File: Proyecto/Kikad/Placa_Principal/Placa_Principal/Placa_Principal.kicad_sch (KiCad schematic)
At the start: 9 parts, among them J1 Screw_Terminal_01x03, J2 Screw_Terminal_01x03, J3 Screw_Terminal_01x03, J4 Screw_Terminal_01x03, J5 USB_C_Receptacle_PowerOnly_6P, J6 Screw_Terminal_01x07, SW1 SW_DIP_x01, U1 ESP32-DEVKITC-32D

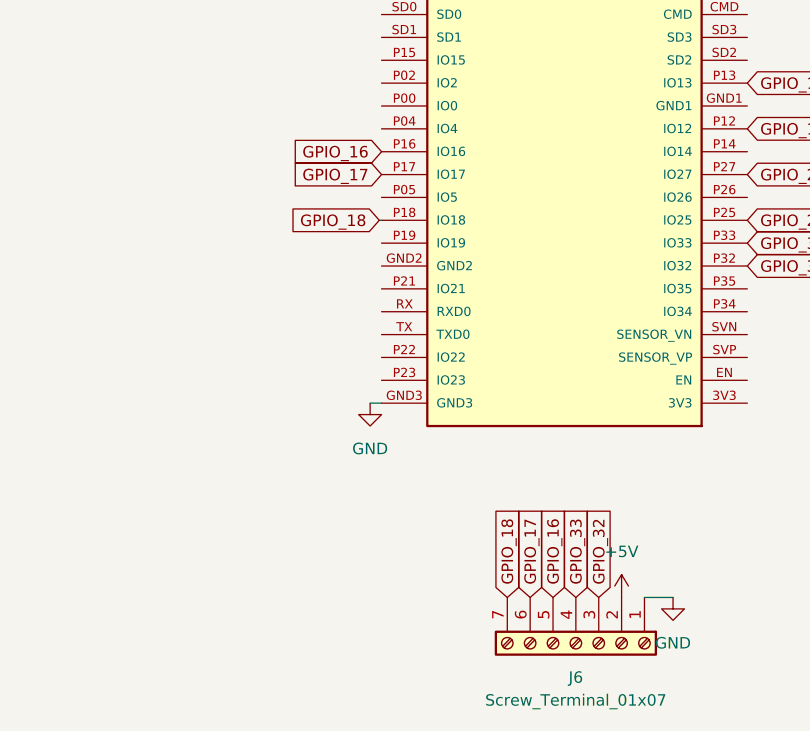
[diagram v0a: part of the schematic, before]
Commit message: Cambie 2 gpio
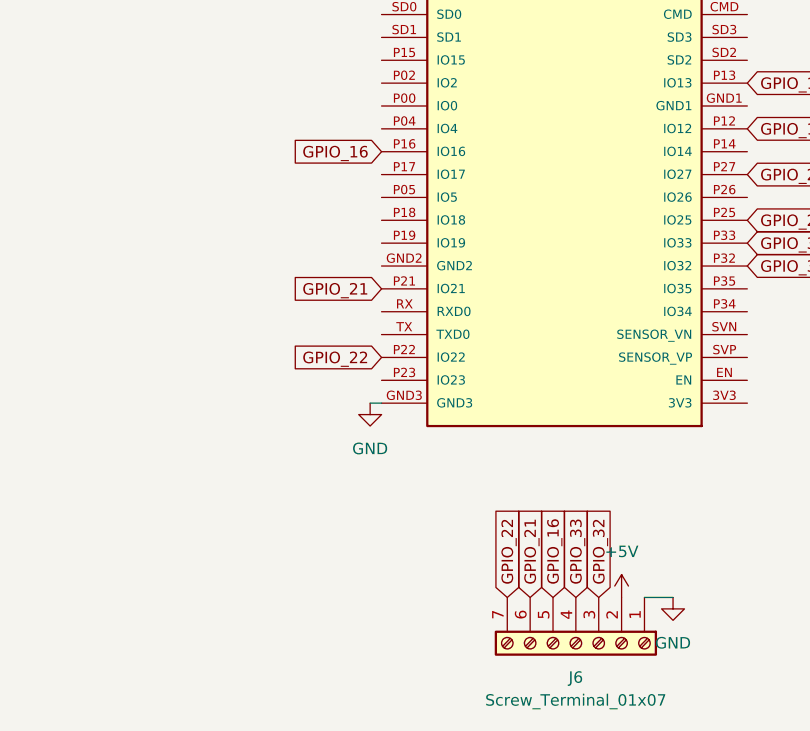
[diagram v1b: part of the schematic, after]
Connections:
- net GPIO_21: now reaches U1.P21 (IO21)
- net GPIO_21: now also J6.6 (Pin_6)
- net GPIO_22: now reaches U1.P22 (IO22)
- net GPIO_22: now also J6.7 (Pin_7)
- net GPIO_17: no longer names the net of U1.P17 (IO17)
- net GPIO_17: no longer J6.6 (Pin_6)
- net GPIO_18: no longer names the net of U1.P18 (IO18)
- net GPIO_18: no longer J6.7 (Pin_7)
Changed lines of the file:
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@@
 	(wire
 		(pts
-			(xy 150.876 106.68) (xy 151.13 106.68)
+			(xy 180.34 148.59) (xy 183.515 148.59)
 		)
 		(stroke
@@
 	(wire
 		(pts
-			(xy 180.34 148.59) (xy 183.515 148.59)
+			(xy 93.98 111.76) (xy 93.98 111.125)
 		)
 		(stroke
@@
 		)
 	)
-	(wire
-		(pts
-			(xy 93.98 111.76) (xy 93.98 111.125)
-		)
-		(stroke
-			(width 0)
-			(type default)
-		)
-	)
 	(global_label "GPIO_12"
 		(shape input)
@@
 		)
 	)
-	(global_label "GPIO_17"
+	(global_label "GPIO_21"
 		(shape input)
 		(at 167.64 148.59 90)
@@
 		)
 	)
-	(global_label "GPIO_18"
+	(global_label "GPIO_22"
 		(shape input)
 		(at 165.1 148.59 90)
@@
 		)
 	)
-	(global_label "GPIO_18"
-		(shape input)
-		(at 150.876 106.68 180)
-		(fields_autoplaced yes)
-		(effects
-			(font
-				(size 1.27 1.27)
-			)
-			(justify right)
-		)
-		(property "Intersheetrefs" "${INTERSHEET_REFS}"
-			(at 140.0289 106.68 0)
+	(global_label "GPIO_22"
+		(shape input)
+		(at 151.13 121.92 180)
+		(fields_autoplaced yes)
+		(effects
+			(font
+				(size 1.27 1.27)
+			)
+			(justify right)
+		)
+		(property "Intersheetrefs" "${INTERSHEET_REFS}"
+			(at 140.2829 121.92 0)
 			(effects
 				(font
@@
 		)
 	)
-	(global_label "GPIO_17"
-		(shape input)
-		(at 151.13 101.6 180)
-		(fields_autoplaced yes)
-		(effects
-			(font
-				(size 1.27 1.27)
-			)
-			(justify right)
-		)
-		(property "Intersheetrefs" "${INTERSHEET_REFS}"
-			(at 140.2829 101.6 0)
-			(effects
-				(font
+	(global_label "GPIO_21"
+		(shape input)
+		(at 151.13 114.3 180)
+		(fields_autoplaced yes)
+		(effects
+			(font
+				(size 1.27 1.27)
+			)
+			(justify right)
+		)
+		(property "Intersheetrefs" "${INTERSHEET_REFS}"
+			(at 140.2829 114.3 0)
+			(effects
+				(font

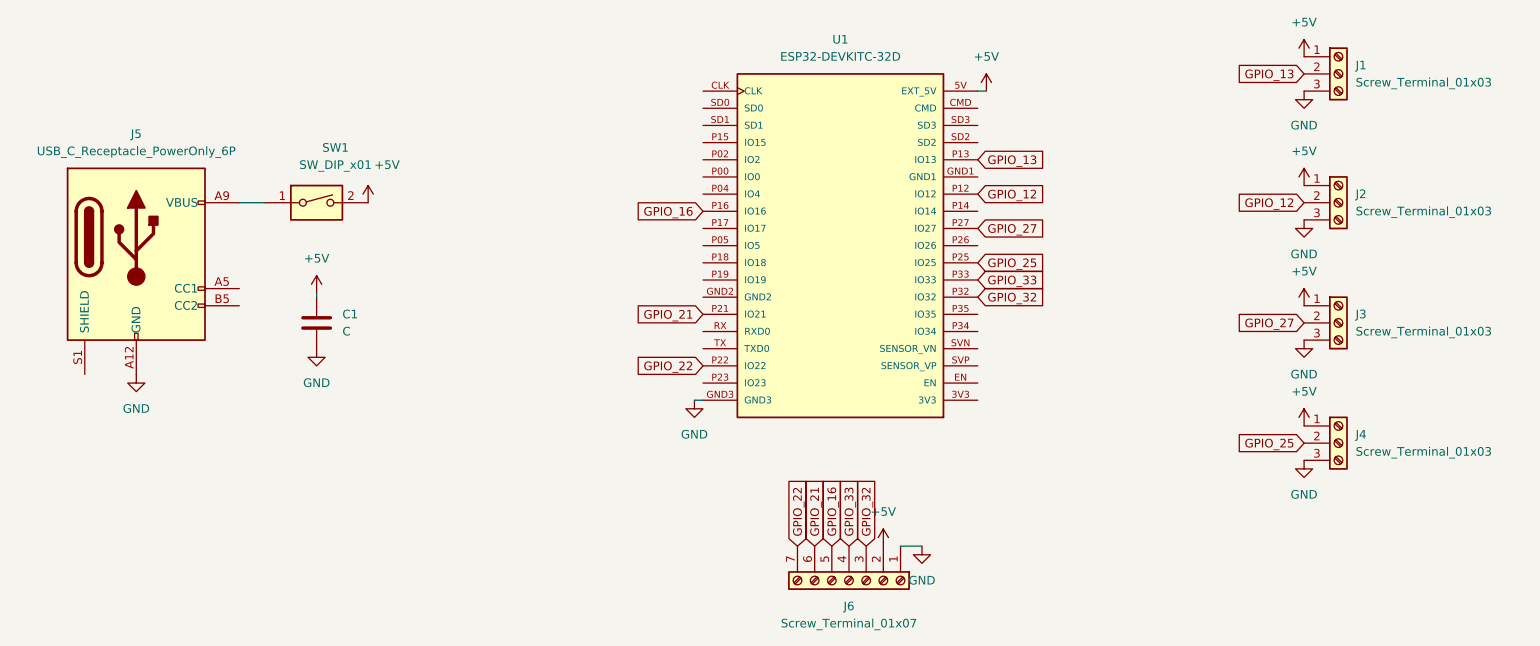
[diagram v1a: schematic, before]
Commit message: Cambie los gpio y agregue un exel
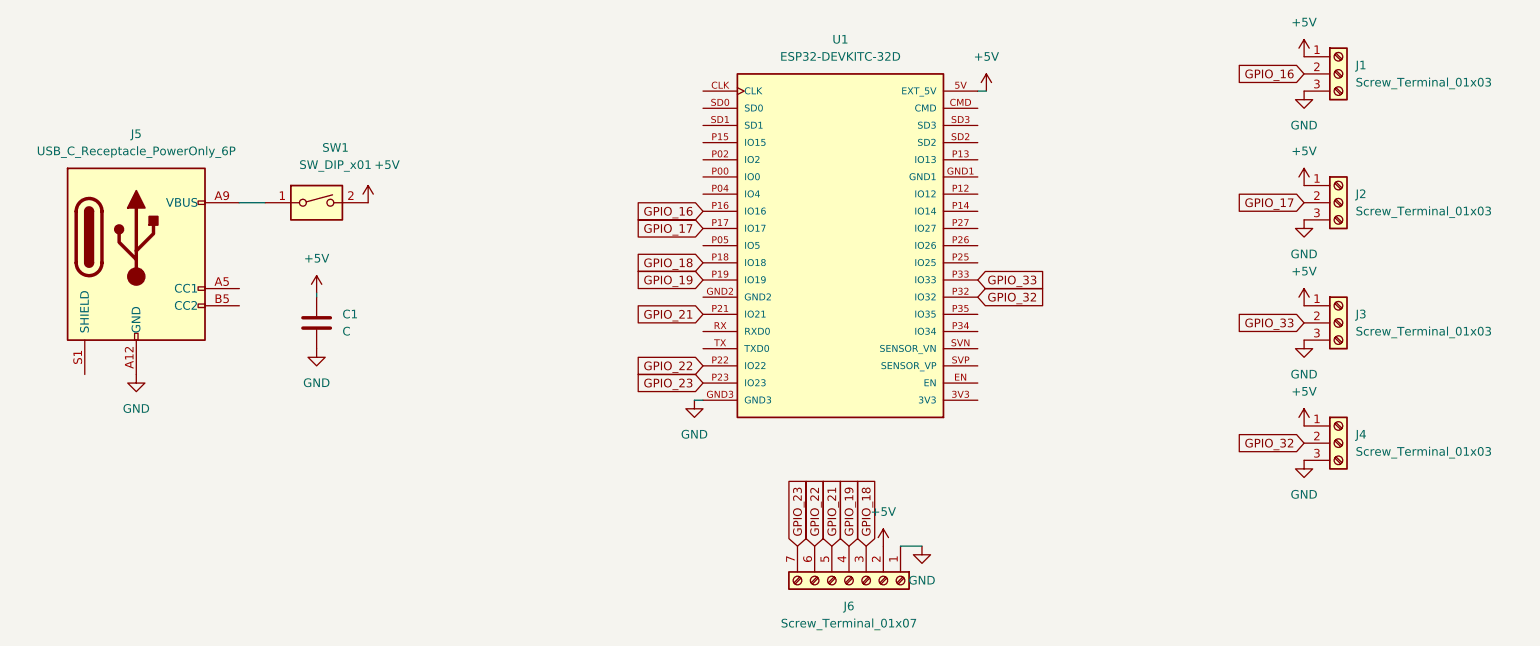
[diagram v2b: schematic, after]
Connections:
- net GPIO_16: now also J1.2 (Pin_2); no longer J6.5 (Pin_5)
- net GPIO_21: now also J6.5 (Pin_5); no longer J6.6 (Pin_6)
- net GPIO_22: now also J6.6 (Pin_6); no longer J6.7 (Pin_7)
- net GPIO_32: now also J4.2 (Pin_2); no longer J6.3 (Pin_3)
- net GPIO_33: now also J3.2 (Pin_2); no longer J6.4 (Pin_4)
- net GPIO_17: now reaches U1.P17 (IO17)
- net GPIO_17: now also J2.2 (Pin_2)
- net GPIO_18: now reaches U1.P18 (IO18)
- net GPIO_18: now also J6.3 (Pin_3)
- net GPIO_19: now reaches U1.P19 (IO19)
- net GPIO_19: now also J6.4 (Pin_4)
- net GPIO_23: now reaches U1.P23 (IO23)
- net GPIO_23: now also J6.7 (Pin_7)
- net GPIO_12: no longer names the net of U1.P12 (IO12)
- net GPIO_12: no longer J2.2 (Pin_2)
- net GPIO_13: no longer names the net of U1.P13 (IO13)
- net GPIO_13: no longer J1.2 (Pin_2)
- net GPIO_25: no longer names the net of U1.P25 (IO25)
- net GPIO_25: no longer J4.2 (Pin_2)
- net GPIO_27: no longer names the net of U1.P27 (IO27)
- net GPIO_27: no longer J3.2 (Pin_2)
